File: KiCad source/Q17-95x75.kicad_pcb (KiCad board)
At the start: 2 copper layers, 96.5 x 76.2 mm, 84 parts, among them J1 TerminalBlock, Q1 IRF610, Q10 2SA970, Q11 BS250, Q12 2SC2240 / AC181, Q13 IRF610, Q14 IRF9610, Q15 FQA46N15, Q16 FQA36P15, Q2 2SA970, Q3 2SC2240, Q4 IRF9610, Q5 IRF9610, Q6 IRF610, Q7 2SC2240, Q8 2N7000, Q9 BS250, U1 DIP-8_W7.62mm_Socket, U1 OPA1641

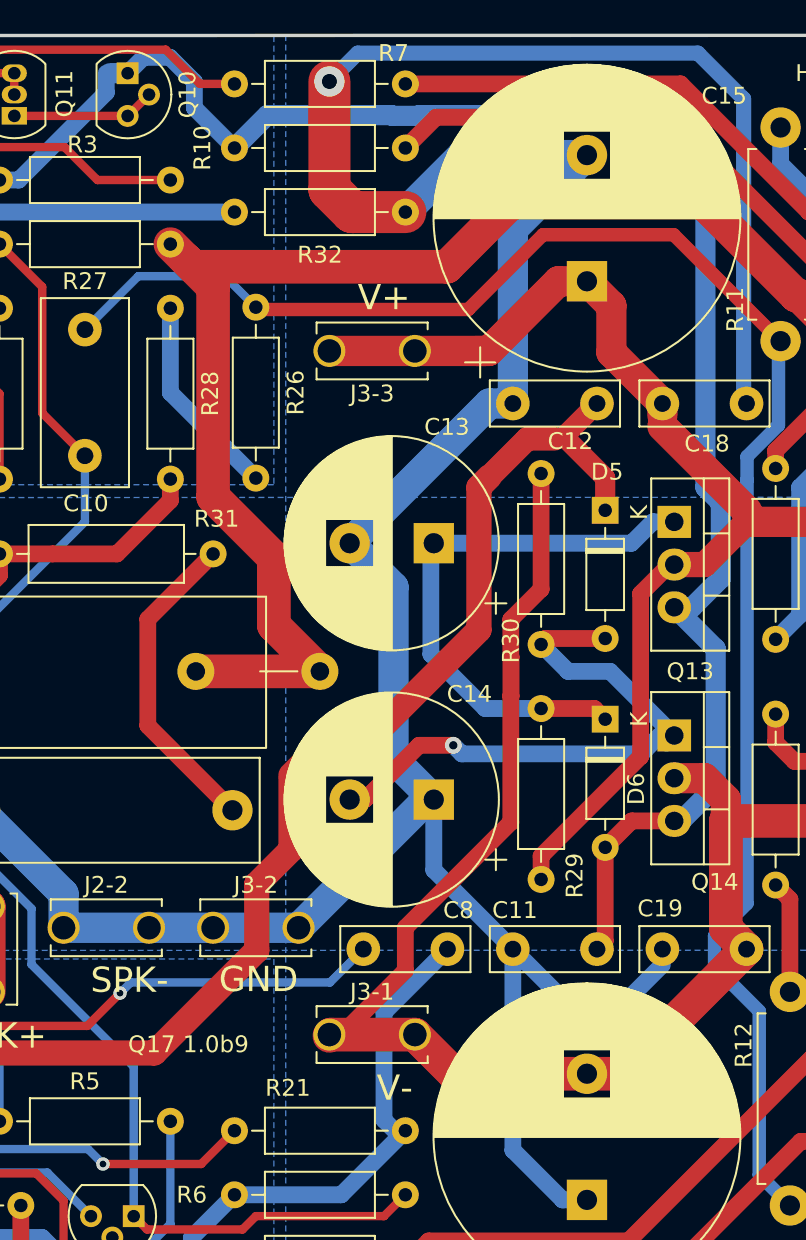
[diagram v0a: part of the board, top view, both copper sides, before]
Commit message: PCB version 1.0b10
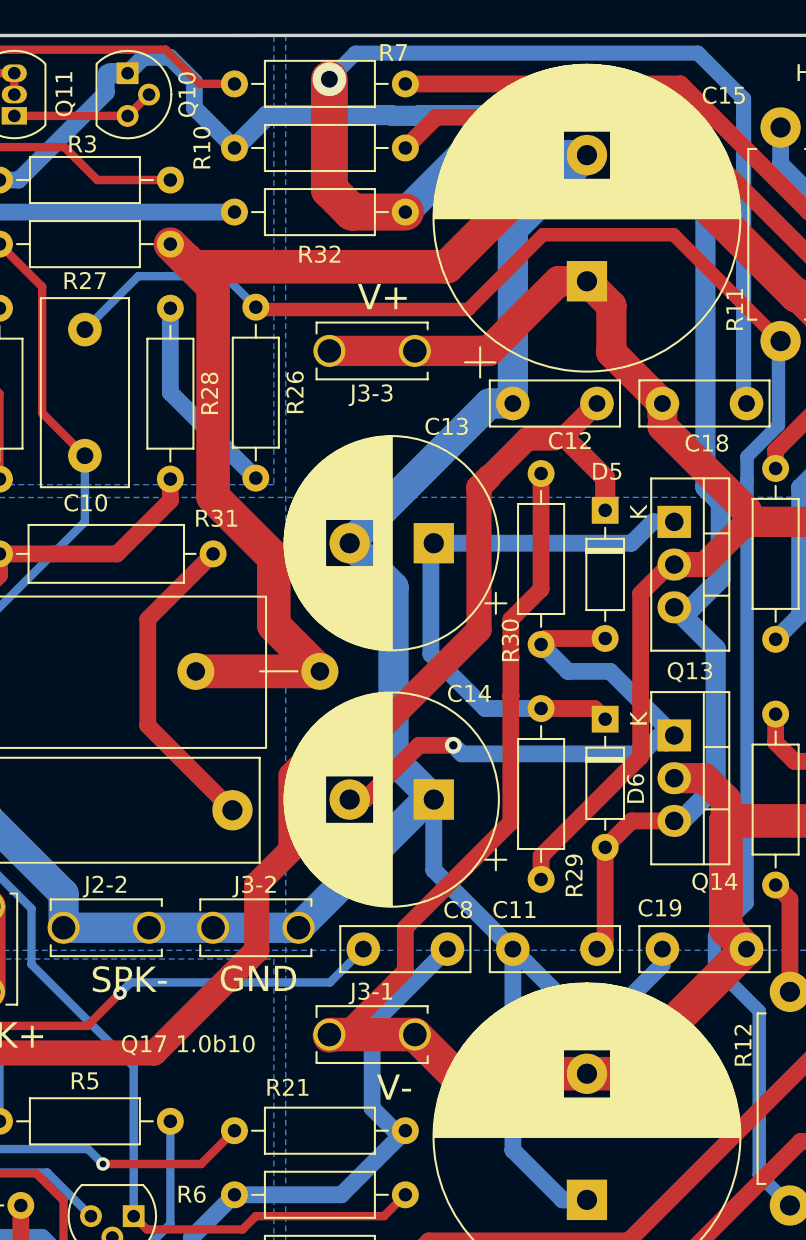
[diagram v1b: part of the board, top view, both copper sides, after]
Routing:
- net GND: track 225.0 -> 225.6 mm
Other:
- board text added: "Q17 1.0b10"
- board text removed: "Q17 1.0b9"
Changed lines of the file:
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@@
     (title "QUAD405 Reborn")
     (date "2021-11-13")
-    (rev "1.0b9")
+    (rev "1.0b10")
     (company "PCB design by Stef")
     (comment 1 "Zize 95 x 75 mm")
@@
     (effects (font (size 0.5 0.5) (thickness 0.125)))
   )
-  (gr_text "Q17 1.0b9" (at 145.288 109.728) (layer "F.SilkS")
+  (gr_text "Q17 1.0b10" (at 145.288 109.728) (layer "F.SilkS")
     (effects (font (size 1 1) (thickness 0.25)))
   )
@@
   (segment (start 120.904 121.661241) (end 120.240952 122.324289) (width 1) (layer "B.Cu") (net 1))
   (segment (start 124.407419 59.6138) (end 127.658619 62.865) (width 1) (layer "B.Cu") (net 1))
-  (segment (start 156.916441 107.8338) (end 160.686441 104.0638) (width 1) (layer "B.Cu") (net 1))
   (segment (start 101.671441 104.0638) (end 103.484118 105.876477) (width 1) (layer "B.Cu") (net 1))
   (segment (start 130.294263 62.865) (end 132.910463 60.2488) (width 1) (layer "B.Cu") (net 1))
-  (segment (start 157.551441 114.8588) (end 156.916441 114.2238) (width 1) (layer "B.Cu") (net 1))
   (segment (start 107.386441 57.7088) (end 107.386441 61.4788) (width 1) (layer "B.Cu") (net 1))
   (segment (start 99.044441 99.860261) (end 101.671441 102.487261) (width 1) (layer "B.Cu") (net 1))
@@
   (segment (start 107.386441 61.4788) (end 111.196441 65.2888) (width 1) (layer "B.Cu") (net 1))
   (segment (start 111.196441 65.2888) (end 109.22 67.265241) (width 1) (layer "B.Cu") (net 1))
+  (segment (start 156.21 108.540241) (end 160.686441 104.0638) (width 1) (layer "B.Cu") (net 1))
   (segment (start 104.085964 84.286477) (end 104.044441 84.328) (width 1) (layer "B.Cu") (net 1))
   (segment (start 144.78 124.46) (end 145.465961 123.774039) (width 1) (layer "B.Cu") (net 1))
@@
   (segment (start 112.466441 84.286477) (end 110.236 86.516918) (width 1) (layer "B.Cu") (net 1))
   (segment (start 145.465961 123.774039) (end 145.465961 121.22928) (width 1) (layer "B.Cu") (net 1))
+  (segment (start 157.551441 114.8588) (end 156.21 113.517359) (width 1) (layer "B.Cu") (net 1))
   (segment (start 148.026441 118.6688) (end 154.376441 118.6688) (width 1) (layer "B.Cu") (net 1))
-  (segment (start 156.916441 114.2238) (end 156.916441 107.8338) (width 1) (layer "B.Cu") (net 1))
   (segment (start 111.196441 65.2888) (end 113.061441 65.2888) (width 1) (layer "B.Cu") (net 1))
   (segment (start 132.910463 60.2488) (end 148.026441 60.2488) (width 1) (layer "B.Cu") (net 1))
@@
   (segment (start 99.044441 99.517281) (end 99.044441 99.860261) (width 0.25) (layer "B.Cu") (net 1))
   (segment (start 158.186441 114.8588) (end 157.551441 114.8588) (width 0.25) (layer "B.Cu") (net 1))
+  (segment (start 156.21 113.517359) (end 156.21 108.540241) (width 1) (layer "B.Cu") (net 1))
   (segment (start 127.658619 62.865) (end 130.294263 62.865) (width 1) (layer "B.Cu") (net 1))
   (segment (start 109.22 81.040036) (end 112.466441 84.286477) (width 1) (layer "B.Cu") (net 1))
@@
   (segment (start 157.354326 54.483) (end 149.982241 54.483) (width 1.2) (layer "B.Cu") (net 12))
   (segment (start 145.6436 52.5018) (end 144.1958 51.054) (width 1) (layer "B.Cu") (net 12))
-  (segment (start 153.67 58.9026) (end 155.0162 60.2488) (width 2.5) (layer "F.Cu") (net 13))
-  (segment (start 153.67 52.4835) (end 153.67 58.9026) (width 2.5) (layer "F.Cu") (net 13))
-  (segment (start 155.0162 60.2488) (end 158.186441 60.2488) (width 2.5) (layer "F.Cu") (net 13))
-  (via (at 153.67 52.4835) (size 1.8) (drill 0.9) (layers "F.Cu" "B.Cu") (free) (net 13))
-  (segment (start 178.292889 71.454448) (end 178.292889 53.515389) (width 0.9) (layer "B.Cu") (net 13))
+  (segment (start 153.669999 52.352791) (end 153.67 58.9026) (width 2.2) (layer "F.Cu") (net 13))
+  (segment (start 155.0162 60.2488) (end 158.186441 60.2488) (width 2.2) (layer "F.Cu") (net 13))
+  (segment (start 153.67 58.9026) (end 155.0162 60.2488) (width 2.2) (layer "F.Cu") (net 13))
+  (via (at 153.669999 52.352791) (size 2) (drill 1) (layers "F.Cu" "B.Cu") (free) (net 13))
   (segment (start 164.576441 104.0638) (end 167.751441 107.2388) (width 1) (layer "B.Cu") (net 13))
-  (segment (start 178.292889 53.515389) (end 175.5775 50.8) (width 0.9) (layer "B.Cu") (net 13))
-  (segment (start 155.3535 50.8) (end 153.67 52.4835) (width 0.9) (layer "B.Cu") (net 13))
+  (segment (start 155.22279 50.8) (end 153.669999 52.352791) (width 0.9) (layer "B.Cu") (net 13))
   (segment (start 159.8754 95.1738) (end 159.8754 99.362759) (width 1) (layer "B.Cu") (net 13))
   (segment (start 159.8754 95.1738) (end 157.48 92.7784) (width 1.8) (layer "B.Cu") (net 13))
@@
   (segment (start 137.866441 102.7938) (end 151.836441 102.7938) (width 1.8) (layer "B.Cu") (net 13))
   (segment (start 168.981441 118.97158) (end 167.531441 118.97158) (width 1) (layer "B.Cu") (net 13))
-  (segment (start 175.5775 50.8) (end 155.3535 50.8) (width 0.9) (layer "B.Cu") (net 13))
+  (segment (start 178.292889 71.454448) (end 178.292889 53.515389) (width 0.9) (layer "B.Cu") (net 13))
   (segment (start 157.48 82.5384) (end 154.8754 79.9338) (width 1.8) (layer "B.Cu") (net 13))
+  (segment (start 178.292889 53.515389) (end 175.5775 50.8) (width 0.9) (layer "B.Cu") (net 13))
   (segment (start 173.466441 104.9963) (end 173.466441 104.0638) (width 0.25) (layer "B.Cu") (net 13))
   (segment (start 157.48 92.7784) (end 157.48 82.5384) (width 1.8) (layer "B.Cu") (net 13))
@@
   (segment (start 137.866441 100.7688) (end 132.906441 95.8088) (width 1.8) (layer "B.Cu") (net 13))
   (segment (start 167.751441 107.2388) (end 171.223941 107.2388) (width 1) (layer "B.Cu") (net 13))
+  (segment (start 175.5775 50.8) (end 155.22279 50.8) (width 0.9) (layer "B.Cu") (net 13))
   (segment (start 137.866441 102.7938) (end 137.866441 100.7688) (width 1.8) (layer "B.Cu") (net 13))
   (segment (start 164.576441 61.26658) (end 168.981441 56.86158) (width 1.8) (layer "B.Cu") (net 13))
